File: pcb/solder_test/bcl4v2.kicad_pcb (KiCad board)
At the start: 2 copper layers, 25.4 x 13.2 mm, 18 parts, among them J1 USB_OTG, J2 Conn_01x05

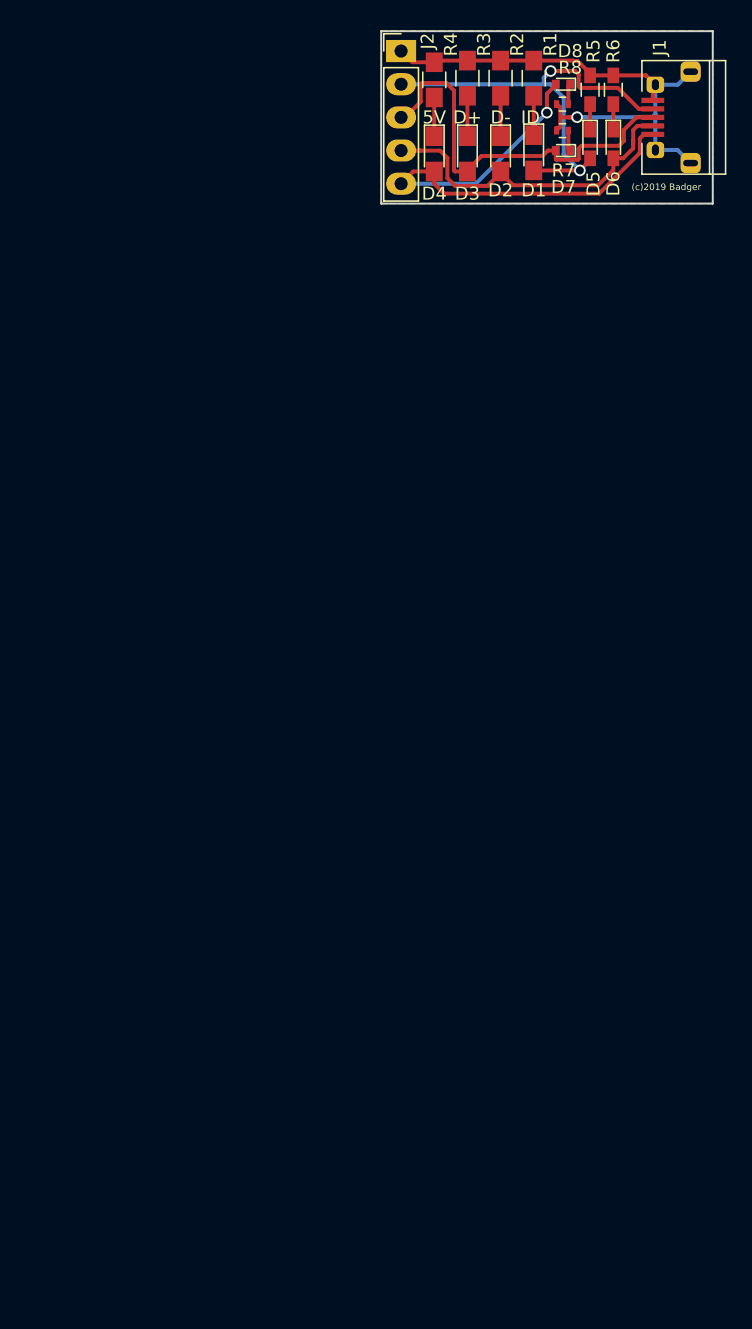
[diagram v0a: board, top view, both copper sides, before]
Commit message: - panelize in design
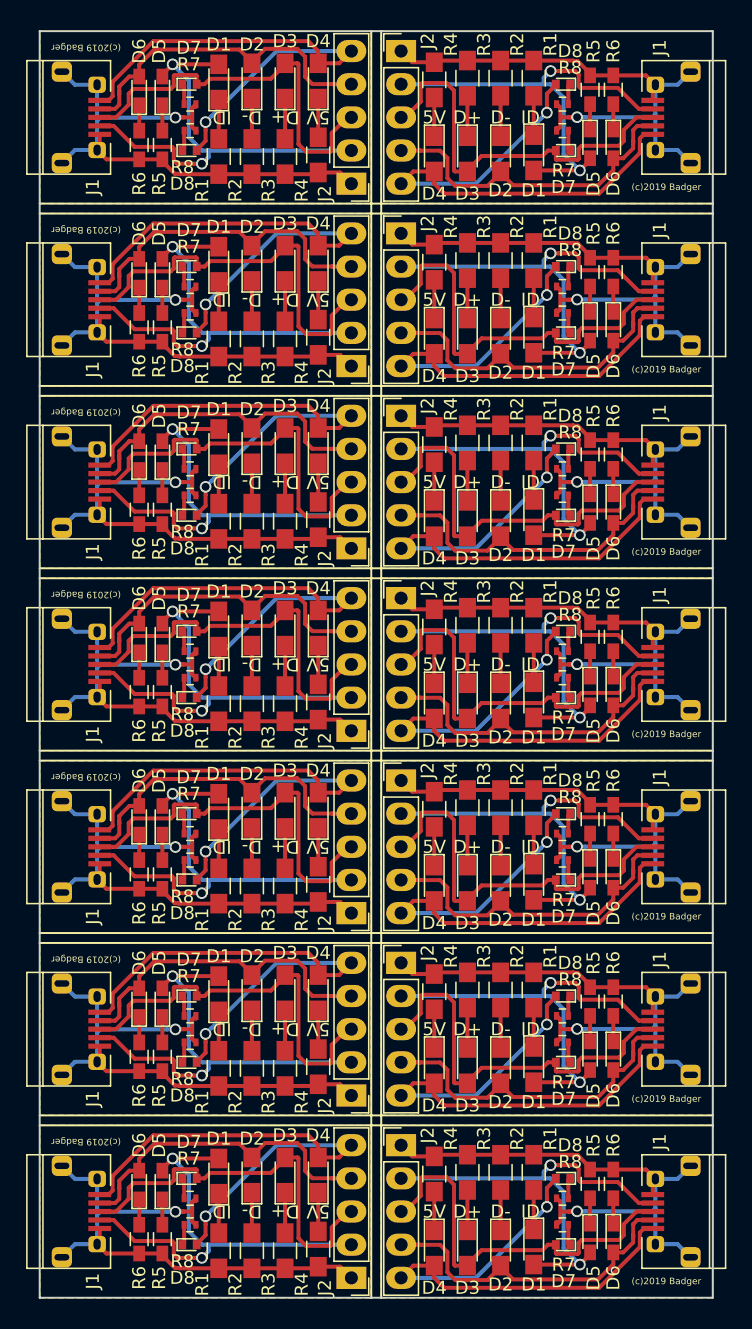
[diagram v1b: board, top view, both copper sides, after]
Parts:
- added D1: LED, LEDs:LED_0805_HandSoldering, F.Cu at (38.9, 58.5)
- added D1: LED, LEDs:LED_0805_HandSoldering, F.Cu at (63.0, 119.8)
- added D1: LED, LEDs:LED_0805_HandSoldering, F.Cu at (63.0, 91.9)
- added D1: LED, LEDs:LED_0805_HandSoldering, F.Cu at (63.0, 77.9)
- added D1: LED, LEDs:LED_0805_HandSoldering, F.Cu at (63.0, 63.9)
- added D1: LED, LEDs:LED_0805_HandSoldering, F.Cu at (38.9, 44.5)
- added D1: LED, LEDs:LED_0805_HandSoldering, F.Cu at (38.9, 86.4)
- added D1: LED, LEDs:LED_0805_HandSoldering, F.Cu at (38.9, 114.4)
- added D1: LED, LEDs:LED_0805_HandSoldering, F.Cu at (38.9, 128.3)
- added D1: LED, LEDs:LED_0805_HandSoldering, F.Cu at (38.9, 100.4)
- added D1: LED, LEDs:LED_0805_HandSoldering, F.Cu at (38.9, 72.5)
- added D1: LED, LEDs:LED_0805_HandSoldering, F.Cu at (63.0, 133.8)
- added D1: LED, LEDs:LED_0805_HandSoldering, F.Cu at (63.0, 105.8)
- added D2: LED, LEDs:LED_0805_HandSoldering, F.Cu at (41.4, 128.3)
- added D2: LED, LEDs:LED_0805_HandSoldering, F.Cu at (60.5, 119.9)
- added D2: LED, LEDs:LED_0805_HandSoldering, F.Cu at (60.5, 78.0)
- added D2: LED, LEDs:LED_0805_HandSoldering, F.Cu at (60.5, 91.9)
- added D2: LED, LEDs:LED_0805_HandSoldering, F.Cu at (60.5, 64.0)
- added D2: LED, LEDs:LED_0805_HandSoldering, F.Cu at (41.4, 86.4)
- added D2: LED, LEDs:LED_0805_HandSoldering, F.Cu at (41.4, 114.3)
- added D2: LED, LEDs:LED_0805_HandSoldering, F.Cu at (41.4, 72.4)
- added D2: LED, LEDs:LED_0805_HandSoldering, F.Cu at (41.4, 100.3)
- added D2: LED, LEDs:LED_0805_HandSoldering, F.Cu at (41.4, 44.5)
- added D2: LED, LEDs:LED_0805_HandSoldering, F.Cu at (41.4, 58.4)
- added D2: LED, LEDs:LED_0805_HandSoldering, F.Cu at (60.5, 133.9)
- added D2: LED, LEDs:LED_0805_HandSoldering, F.Cu at (60.5, 105.9)
- added D3: LED, LEDs:LED_0805_HandSoldering, F.Cu at (43.9, 100.3)
- added D3: LED, LEDs:LED_0805_HandSoldering, F.Cu at (57.9, 133.9)
- added D3: LED, LEDs:LED_0805_HandSoldering, F.Cu at (57.9, 91.9)
- added D3: LED, LEDs:LED_0805_HandSoldering, F.Cu at (57.9, 78.0)
- added D3: LED, LEDs:LED_0805_HandSoldering, F.Cu at (57.9, 64.0)
- added D3: LED, LEDs:LED_0805_HandSoldering, F.Cu at (43.9, 72.4)
- added D3: LED, LEDs:LED_0805_HandSoldering, F.Cu at (43.9, 114.3)
- added D3: LED, LEDs:LED_0805_HandSoldering, F.Cu at (43.9, 128.3)
- added D3: LED, LEDs:LED_0805_HandSoldering, F.Cu at (43.9, 86.4)
- added D3: LED, LEDs:LED_0805_HandSoldering, F.Cu at (43.9, 44.5)
- added D3: LED, LEDs:LED_0805_HandSoldering, F.Cu at (43.9, 58.4)
- added D3: LED, LEDs:LED_0805_HandSoldering, F.Cu at (57.9, 119.9)
- added D3: LED, LEDs:LED_0805_HandSoldering, F.Cu at (57.9, 105.9)
- added D4: LED, LEDs:LED_0805_HandSoldering, F.Cu at (46.5, 86.4)
- added D4: LED, LEDs:LED_0805_HandSoldering, F.Cu at (55.4, 105.9)
- added D4: LED, LEDs:LED_0805_HandSoldering, F.Cu at (55.4, 91.9)
- added D4: LED, LEDs:LED_0805_HandSoldering, F.Cu at (55.4, 78.0)
- added D4: LED, LEDs:LED_0805_HandSoldering, F.Cu at (55.4, 64.0)
- added D4: LED, LEDs:LED_0805_HandSoldering, F.Cu at (46.5, 58.4)
- added D4: LED, LEDs:LED_0805_HandSoldering, F.Cu at (46.5, 44.5)
- added D4: LED, LEDs:LED_0805_HandSoldering, F.Cu at (46.5, 72.4)
- added D4: LED, LEDs:LED_0805_HandSoldering, F.Cu at (46.5, 100.3)
- added D4: LED, LEDs:LED_0805_HandSoldering, F.Cu at (46.5, 114.3)
- added D4: LED, LEDs:LED_0805_HandSoldering, F.Cu at (46.5, 128.3)
- added D4: LED, LEDs:LED_0805_HandSoldering, F.Cu at (55.4, 133.9)
- added D4: LED, LEDs:LED_0805_HandSoldering, F.Cu at (55.4, 119.9)
- added D5: LED, LEDs:LED_0603_HandSoldering, F.Cu at (34.5, 115.1)
- added D5: LED, LEDs:LED_0603_HandSoldering, F.Cu at (67.3, 119.1)
- added D5: LED, LEDs:LED_0603_HandSoldering, F.Cu at (67.3, 91.2)
- added D5: LED, LEDs:LED_0603_HandSoldering, F.Cu at (67.3, 77.2)
- added D5: LED, LEDs:LED_0603_HandSoldering, F.Cu at (67.3, 63.2)
- added D5: LED, LEDs:LED_0603_HandSoldering, F.Cu at (34.5, 45.2)
- added D5: LED, LEDs:LED_0603_HandSoldering, F.Cu at (34.5, 87.1)
- added D5: LED, LEDs:LED_0603_HandSoldering, F.Cu at (34.5, 101.1)
- added D5: LED, LEDs:LED_0603_HandSoldering, F.Cu at (34.5, 59.2)
- added D5: LED, LEDs:LED_0603_HandSoldering, F.Cu at (34.5, 73.2)
- added D5: LED, LEDs:LED_0603_HandSoldering, F.Cu at (34.5, 129.0)
- added D5: LED, LEDs:LED_0603_HandSoldering, F.Cu at (67.3, 105.2)
- added D5: LED, LEDs:LED_0603_HandSoldering, F.Cu at (67.3, 133.1)
- added D6: LED, LEDs:LED_0603_HandSoldering, F.Cu at (32.8, 59.2)
- added D6: LED, LEDs:LED_0603_HandSoldering, F.Cu at (69.1, 133.1)
- added D6: LED, LEDs:LED_0603_HandSoldering, F.Cu at (69.1, 91.2)
- added D6: LED, LEDs:LED_0603_HandSoldering, F.Cu at (69.1, 77.2)
- added D6: LED, LEDs:LED_0603_HandSoldering, F.Cu at (69.1, 63.2)
- added D6: LED, LEDs:LED_0603_HandSoldering, F.Cu at (32.8, 101.1)
- added D6: LED, LEDs:LED_0603_HandSoldering, F.Cu at (32.8, 115.1)
- added D6: LED, LEDs:LED_0603_HandSoldering, F.Cu at (32.8, 73.2)
- added D6: LED, LEDs:LED_0603_HandSoldering, F.Cu at (32.8, 87.1)
- added D6: LED, LEDs:LED_0603_HandSoldering, F.Cu at (32.8, 129.0)
- added D6: LED, LEDs:LED_0603_HandSoldering, F.Cu at (32.8, 45.2)
- added D6: LED, LEDs:LED_0603_HandSoldering, F.Cu at (69.1, 119.1)
- added D6: LED, LEDs:LED_0603_HandSoldering, F.Cu at (69.1, 105.2)
- added D7: LED, LEDs:LED_0402, F.Cu at (36.6, 44.7)
- added D7: LED, LEDs:LED_0402, F.Cu at (65.2, 119.6)
- added D7: LED, LEDs:LED_0402, F.Cu at (65.2, 91.7)
- added D7: LED, LEDs:LED_0402, F.Cu at (65.2, 77.7)
- added D7: LED, LEDs:LED_0402, F.Cu at (65.2, 63.8)
- added D7: LED, LEDs:LED_0402, F.Cu at (36.6, 114.6)
- added D7: LED, LEDs:LED_0402, F.Cu at (36.6, 128.5)
- added D7: LED, LEDs:LED_0402, F.Cu at (36.6, 72.6)
- added D7: LED, LEDs:LED_0402, F.Cu at (36.6, 86.6)
- added D7: LED, LEDs:LED_0402, F.Cu at (36.6, 58.7)
- added D7: LED, LEDs:LED_0402, F.Cu at (36.6, 100.6)
- added D7: LED, LEDs:LED_0402, F.Cu at (65.2, 105.7)
- added D7: LED, LEDs:LED_0402, F.Cu at (65.2, 133.6)
- added D8: LED, LEDs:LED_0402, F.Cu at (36.6, 119.6)
- added D8: LED, LEDs:LED_0402, F.Cu at (65.2, 114.6)
- added D8: LED, LEDs:LED_0402, F.Cu at (65.2, 86.6)
- added D8: LED, LEDs:LED_0402, F.Cu at (65.2, 72.6)
- added D8: LED, LEDs:LED_0402, F.Cu at (65.2, 58.7)
- added D8: LED, LEDs:LED_0402, F.Cu at (36.6, 91.7)
- added D8: LED, LEDs:LED_0402, F.Cu at (36.6, 49.8)
- added D8: LED, LEDs:LED_0402, F.Cu at (36.6, 77.7)
- added D8: LED, LEDs:LED_0402, F.Cu at (36.6, 133.6)
- added D8: LED, LEDs:LED_0402, F.Cu at (36.6, 63.8)
- added D8: LED, LEDs:LED_0402, F.Cu at (36.6, 105.7)
- added D8: LED, LEDs:LED_0402, F.Cu at (65.2, 100.6)
- added D8: LED, LEDs:LED_0402, F.Cu at (65.2, 128.5)
- added J1: USB_OTG, kicad_libraries_new:badger_USB_Micro-B_handsolder, F.Cu at (28.2, 89.2)
- added J1: USB_OTG, kicad_libraries_new:badger_USB_Micro-B_handsolder, F.Cu at (73.7, 117.1)
- added J1: USB_OTG, kicad_libraries_new:badger_USB_Micro-B_handsolder, F.Cu at (73.7, 75.2)
- added J1: USB_OTG, kicad_libraries_new:badger_USB_Micro-B_handsolder, F.Cu at (73.7, 89.2)
- added J1: USB_OTG, kicad_libraries_new:badger_USB_Micro-B_handsolder, F.Cu at (73.7, 61.2)
- added J1: USB_OTG, kicad_libraries_new:badger_USB_Micro-B_handsolder, F.Cu at (28.2, 47.2)
- added J1: USB_OTG, kicad_libraries_new:badger_USB_Micro-B_handsolder, F.Cu at (28.2, 131.1)
- added J1: USB_OTG, kicad_libraries_new:badger_USB_Micro-B_handsolder, F.Cu at (28.2, 117.1)
- added J1: USB_OTG, kicad_libraries_new:badger_USB_Micro-B_handsolder, F.Cu at (28.2, 61.2)
- added J1: USB_OTG, kicad_libraries_new:badger_USB_Micro-B_handsolder, F.Cu at (28.2, 103.1)
- added J1: USB_OTG, kicad_libraries_new:badger_USB_Micro-B_handsolder, F.Cu at (28.2, 75.2)
- added J1: USB_OTG, kicad_libraries_new:badger_USB_Micro-B_handsolder, F.Cu at (73.7, 131.1)
- added J1: USB_OTG, kicad_libraries_new:badger_USB_Micro-B_handsolder, F.Cu at (73.7, 103.1)
- added J2: Conn_01x05, kicad_libraries_new:badger_Pin_Hdr_1x05_2.54mm_handsolder, F.Cu at (49.0, 80.3)
- added J2: Conn_01x05, kicad_libraries_new:badger_Pin_Hdr_1x05_2.54mm_handsolder, F.Cu at (52.8, 98.0)
- added J2: Conn_01x05, kicad_libraries_new:badger_Pin_Hdr_1x05_2.54mm_handsolder, F.Cu at (52.8, 84.1)
- added J2: Conn_01x05, kicad_libraries_new:badger_Pin_Hdr_1x05_2.54mm_handsolder, F.Cu at (52.8, 70.1)
- added J2: Conn_01x05, kicad_libraries_new:badger_Pin_Hdr_1x05_2.54mm_handsolder, F.Cu at (52.8, 56.1)
- added J2: Conn_01x05, kicad_libraries_new:badger_Pin_Hdr_1x05_2.54mm_handsolder, F.Cu at (49.0, 52.3)
- added J2: Conn_01x05, kicad_libraries_new:badger_Pin_Hdr_1x05_2.54mm_handsolder, F.Cu at (49.0, 108.2)
- added J2: Conn_01x05, kicad_libraries_new:badger_Pin_Hdr_1x05_2.54mm_handsolder, F.Cu at (49.0, 94.2)
- added J2: Conn_01x05, kicad_libraries_new:badger_Pin_Hdr_1x05_2.54mm_handsolder, F.Cu at (49.0, 122.2)
- added J2: Conn_01x05, kicad_libraries_new:badger_Pin_Hdr_1x05_2.54mm_handsolder, F.Cu at (49.0, 66.3)
- added J2: Conn_01x05, kicad_libraries_new:badger_Pin_Hdr_1x05_2.54mm_handsolder, F.Cu at (49.0, 136.1)
- added J2: Conn_01x05, kicad_libraries_new:badger_Pin_Hdr_1x05_2.54mm_handsolder, F.Cu at (52.8, 112.0)
- added J2: Conn_01x05, kicad_libraries_new:badger_Pin_Hdr_1x05_2.54mm_handsolder, F.Cu at (52.8, 126.0)
- added R1: 1k, Resistors_SMD:R_0805_HandSoldering, F.Cu at (38.9, 120.1)
- added R1: 1k, Resistors_SMD:R_0805_HandSoldering, F.Cu at (63.0, 128.1)
- added R1: 1k, Resistors_SMD:R_0805_HandSoldering, F.Cu at (63.0, 86.2)
- added R1: 1k, Resistors_SMD:R_0805_HandSoldering, F.Cu at (63.0, 72.2)
- added R1: 1k, Resistors_SMD:R_0805_HandSoldering, F.Cu at (63.0, 58.2)
- added R1: 1k, Resistors_SMD:R_0805_HandSoldering, F.Cu at (38.9, 50.2)
- added R1: 1k, Resistors_SMD:R_0805_HandSoldering, F.Cu at (38.9, 106.1)
- added R1: 1k, Resistors_SMD:R_0805_HandSoldering, F.Cu at (38.9, 92.2)
- added R1: 1k, Resistors_SMD:R_0805_HandSoldering, F.Cu at (38.9, 64.2)
- added R1: 1k, Resistors_SMD:R_0805_HandSoldering, F.Cu at (38.9, 78.2)
- added R1: 1k, Resistors_SMD:R_0805_HandSoldering, F.Cu at (38.9, 134.1)
- added R1: 1k, Resistors_SMD:R_0805_HandSoldering, F.Cu at (63.0, 100.1)
- added R1: 1k, Resistors_SMD:R_0805_HandSoldering, F.Cu at (63.0, 114.1)
- added R2: 1k, Resistors_SMD:R_0805_HandSoldering, F.Cu at (41.4, 106.1)
- added R2: 1k, Resistors_SMD:R_0805_HandSoldering, F.Cu at (60.5, 128.1)
- added R2: 1k, Resistors_SMD:R_0805_HandSoldering, F.Cu at (60.5, 86.2)
- added R2: 1k, Resistors_SMD:R_0805_HandSoldering, F.Cu at (60.5, 72.2)
- added R2: 1k, Resistors_SMD:R_0805_HandSoldering, F.Cu at (60.5, 58.2)
- added R2: 1k, Resistors_SMD:R_0805_HandSoldering, F.Cu at (41.4, 120.1)
- added R2: 1k, Resistors_SMD:R_0805_HandSoldering, F.Cu at (41.4, 64.2)
- added R2: 1k, Resistors_SMD:R_0805_HandSoldering, F.Cu at (41.4, 78.2)
- added R2: 1k, Resistors_SMD:R_0805_HandSoldering, F.Cu at (41.4, 134.1)
- added R2: 1k, Resistors_SMD:R_0805_HandSoldering, F.Cu at (41.4, 92.2)
- added R2: 1k, Resistors_SMD:R_0805_HandSoldering, F.Cu at (41.4, 50.2)
- added R2: 1k, Resistors_SMD:R_0805_HandSoldering, F.Cu at (60.5, 114.1)
- added R2: 1k, Resistors_SMD:R_0805_HandSoldering, F.Cu at (60.5, 100.1)
- added R3: 1k, Resistors_SMD:R_0805_HandSoldering, F.Cu at (43.9, 120.1)
- added R3: 1k, Resistors_SMD:R_0805_HandSoldering, F.Cu at (57.9, 128.1)
- added R3: 1k, Resistors_SMD:R_0805_HandSoldering, F.Cu at (57.9, 86.2)
- added R3: 1k, Resistors_SMD:R_0805_HandSoldering, F.Cu at (57.9, 72.2)
- added R3: 1k, Resistors_SMD:R_0805_HandSoldering, F.Cu at (57.9, 58.2)
- added R3: 1k, Resistors_SMD:R_0805_HandSoldering, F.Cu at (43.9, 106.1)
- added R3: 1k, Resistors_SMD:R_0805_HandSoldering, F.Cu at (43.9, 78.2)
- added R3: 1k, Resistors_SMD:R_0805_HandSoldering, F.Cu at (43.9, 92.2)
- added R3: 1k, Resistors_SMD:R_0805_HandSoldering, F.Cu at (43.9, 50.2)
- added R3: 1k, Resistors_SMD:R_0805_HandSoldering, F.Cu at (43.9, 64.2)
- added R3: 1k, Resistors_SMD:R_0805_HandSoldering, F.Cu at (43.9, 134.1)
- added R3: 1k, Resistors_SMD:R_0805_HandSoldering, F.Cu at (57.9, 100.1)
- added R3: 1k, Resistors_SMD:R_0805_HandSoldering, F.Cu at (57.9, 114.1)
- added R4: 1k, Resistors_SMD:R_0805_HandSoldering, F.Cu at (46.5, 120.0)
- added R4: 1k, Resistors_SMD:R_0805_HandSoldering, F.Cu at (55.4, 114.2)
- added R4: 1k, Resistors_SMD:R_0805_HandSoldering, F.Cu at (55.4, 86.3)
- added R4: 1k, Resistors_SMD:R_0805_HandSoldering, F.Cu at (55.4, 72.3)
- added R4: 1k, Resistors_SMD:R_0805_HandSoldering, F.Cu at (55.4, 58.3)
- added R4: 1k, Resistors_SMD:R_0805_HandSoldering, F.Cu at (46.5, 133.9)
- added R4: 1k, Resistors_SMD:R_0805_HandSoldering, F.Cu at (46.5, 92.0)
- added R4: 1k, Resistors_SMD:R_0805_HandSoldering, F.Cu at (46.5, 64.1)
- added R4: 1k, Resistors_SMD:R_0805_HandSoldering, F.Cu at (46.5, 106.0)
- added R4: 1k, Resistors_SMD:R_0805_HandSoldering, F.Cu at (46.5, 50.1)
- added R4: 1k, Resistors_SMD:R_0805_HandSoldering, F.Cu at (46.5, 78.1)
- added R4: 1k, Resistors_SMD:R_0805_HandSoldering, F.Cu at (55.4, 100.2)
- added R4: 1k, Resistors_SMD:R_0805_HandSoldering, F.Cu at (55.4, 128.2)
- added R5: 1k, Resistors_SMD:R_0603_HandSoldering, F.Cu at (34.5, 119.2)
- added R5: 1k, Resistors_SMD:R_0603_HandSoldering, F.Cu at (67.3, 115.0)
- added R5: 1k, Resistors_SMD:R_0603_HandSoldering, F.Cu at (67.3, 87.0)
- added R5: 1k, Resistors_SMD:R_0603_HandSoldering, F.Cu at (67.3, 73.1)
- added R5: 1k, Resistors_SMD:R_0603_HandSoldering, F.Cu at (67.3, 59.1)
- added R5: 1k, Resistors_SMD:R_0603_HandSoldering, F.Cu at (34.5, 63.3)
- added R5: 1k, Resistors_SMD:R_0603_HandSoldering, F.Cu at (34.5, 49.4)
- added R5: 1k, Resistors_SMD:R_0603_HandSoldering, F.Cu at (34.5, 91.3)
- added R5: 1k, Resistors_SMD:R_0603_HandSoldering, F.Cu at (34.5, 105.2)
- added R5: 1k, Resistors_SMD:R_0603_HandSoldering, F.Cu at (34.5, 133.2)
- added R5: 1k, Resistors_SMD:R_0603_HandSoldering, F.Cu at (34.5, 77.3)
- added R5: 1k, Resistors_SMD:R_0603_HandSoldering, F.Cu at (67.3, 101.0)
- added R5: 1k, Resistors_SMD:R_0603_HandSoldering, F.Cu at (67.3, 128.9)
- added R6: 1k, Resistors_SMD:R_0603_HandSoldering, F.Cu at (32.8, 105.2)
- added R6: 1k, Resistors_SMD:R_0603_HandSoldering, F.Cu at (69.1, 128.9)
- added R6: 1k, Resistors_SMD:R_0603_HandSoldering, F.Cu at (69.1, 87.0)
- added R6: 1k, Resistors_SMD:R_0603_HandSoldering, F.Cu at (69.1, 73.1)
- added R6: 1k, Resistors_SMD:R_0603_HandSoldering, F.Cu at (69.1, 59.1)
- added R6: 1k, Resistors_SMD:R_0603_HandSoldering, F.Cu at (32.8, 77.3)
- added R6: 1k, Resistors_SMD:R_0603_HandSoldering, F.Cu at (32.8, 49.4)
- added R6: 1k, Resistors_SMD:R_0603_HandSoldering, F.Cu at (32.8, 119.2)
- added R6: 1k, Resistors_SMD:R_0603_HandSoldering, F.Cu at (32.8, 133.2)
- added R6: 1k, Resistors_SMD:R_0603_HandSoldering, F.Cu at (32.8, 91.3)
- added R6: 1k, Resistors_SMD:R_0603_HandSoldering, F.Cu at (32.8, 63.3)
- added R6: 1k, Resistors_SMD:R_0603_HandSoldering, F.Cu at (69.1, 115.0)
- added R6: 1k, Resistors_SMD:R_0603_HandSoldering, F.Cu at (69.1, 101.0)
- added R7: 1k, Resistors_SMD:R_0402, F.Cu at (36.7, 116.1)
- added R7: 1k, Resistors_SMD:R_0402, F.Cu at (65.2, 118.1)
- added R7: 1k, Resistors_SMD:R_0402, F.Cu at (65.2, 90.2)
- added R7: 1k, Resistors_SMD:R_0402, F.Cu at (65.2, 76.2)
- added R7: 1k, Resistors_SMD:R_0402, F.Cu at (65.2, 62.2)
- added R7: 1k, Resistors_SMD:R_0402, F.Cu at (36.7, 88.1)
- added R7: 1k, Resistors_SMD:R_0402, F.Cu at (36.7, 130.0)
- added R7: 1k, Resistors_SMD:R_0402, F.Cu at (36.7, 102.1)
- added R7: 1k, Resistors_SMD:R_0402, F.Cu at (36.7, 46.2)
- added R7: 1k, Resistors_SMD:R_0402, F.Cu at (36.7, 60.2)
- added R7: 1k, Resistors_SMD:R_0402, F.Cu at (36.7, 74.2)
- added R7: 1k, Resistors_SMD:R_0402, F.Cu at (65.2, 104.1)
- added R7: 1k, Resistors_SMD:R_0402, F.Cu at (65.2, 132.1)
- added R8: 1k, Resistors_SMD:R_0402, F.Cu at (36.7, 104.1)
- added R8: 1k, Resistors_SMD:R_0402, F.Cu at (65.2, 102.1)
- added R8: 1k, Resistors_SMD:R_0402, F.Cu at (65.2, 74.2)
- added R8: 1k, Resistors_SMD:R_0402, F.Cu at (65.2, 88.1)
- added R8: 1k, Resistors_SMD:R_0402, F.Cu at (65.2, 60.2)
- added R8: 1k, Resistors_SMD:R_0402, F.Cu at (36.7, 90.2)
- added R8: 1k, Resistors_SMD:R_0402, F.Cu at (36.7, 62.2)
- added R8: 1k, Resistors_SMD:R_0402, F.Cu at (36.7, 76.2)
- added R8: 1k, Resistors_SMD:R_0402, F.Cu at (36.7, 132.1)
- added R8: 1k, Resistors_SMD:R_0402, F.Cu at (36.7, 118.1)
- added R8: 1k, Resistors_SMD:R_0402, F.Cu at (36.7, 48.3)
- added R8: 1k, Resistors_SMD:R_0402, F.Cu at (65.2, 116.1)
- added R8: 1k, Resistors_SMD:R_0402, F.Cu at (65.2, 130.0)
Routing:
- net GND: track 43.7 -> 612.3 mm, vias 1 -> 14
- net +5V: track 39.3 -> 550.6 mm, vias 1 -> 14
- net /ID: track 34.5 -> 483.5 mm, vias 2 -> 28
- net /D+: track 31.4 -> 438.9 mm
- net /D-: track 25.8 -> 361.2 mm
- net Net-(D1-Pad1): track 4.27 -> 59.7 mm
- net Net-(D3-Pad1): track 3.09 -> 43.3 mm
- net Net-(D2-Pad1): track 3.09 -> 43.3 mm
- net Net-(D4-Pad1): track 2.97 -> 41.6 mm
- net Net-(D6-Pad1): track 1.95 -> 27.3 mm
- net Net-(D5-Pad1): track 1.95 -> 27.3 mm
- net Net-(D7-Pad1): track 1.77 -> 24.8 mm
- net Net-(D8-Pad1): track 1.58 -> 22.2 mm
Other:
- board size 25.4 x 13.2 mm -> 51.6 x 97 mm
